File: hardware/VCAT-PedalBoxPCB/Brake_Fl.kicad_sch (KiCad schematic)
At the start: 7 parts, among them U4 INA241A5xD

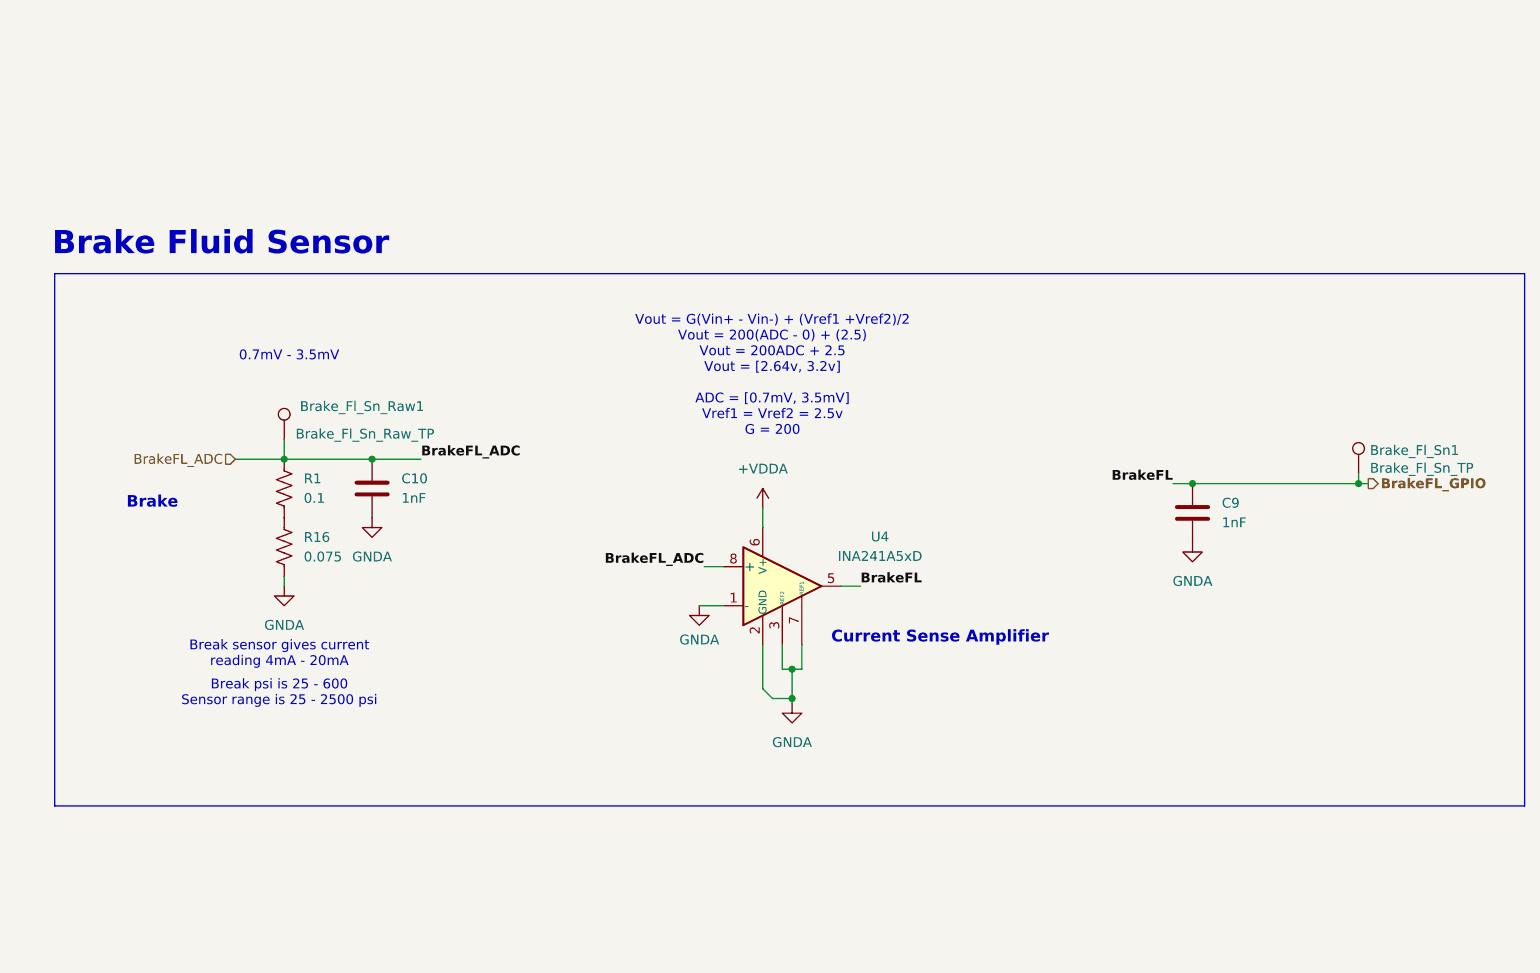
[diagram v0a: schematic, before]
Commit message: Rev B - Initial Layout
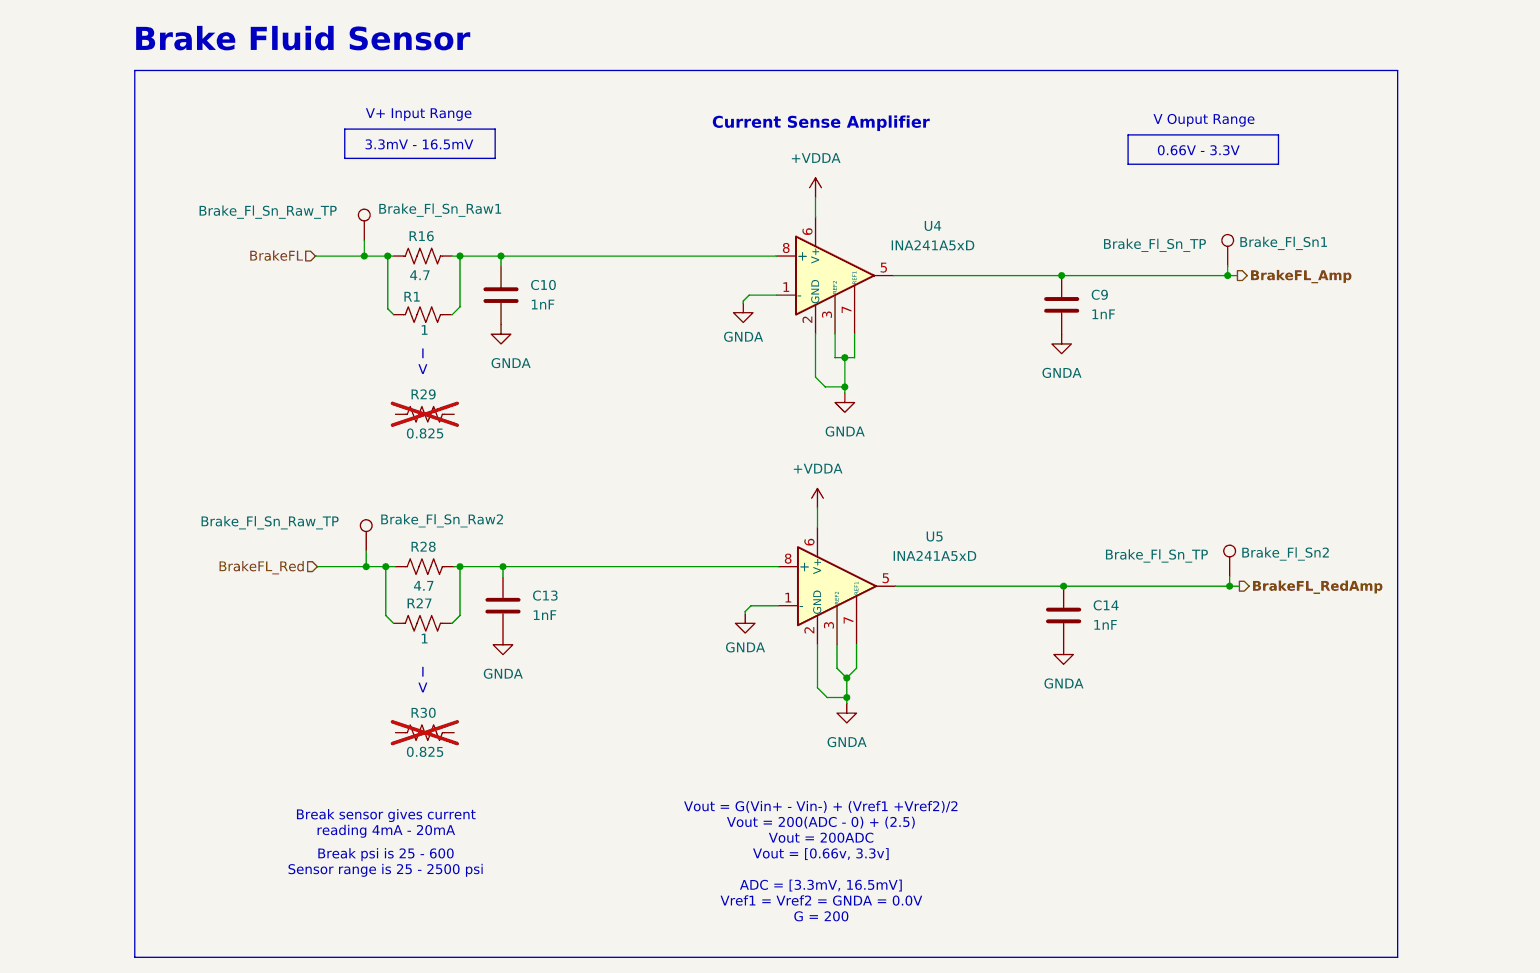
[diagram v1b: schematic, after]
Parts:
- added Brake_Fl_Sn2: Brake_Fl_Sn_TP, TestPoint:TestPoint_THTPad_1.5x1.5mm_Drill0.7mm, symbol Connector:TestPoint
- added Brake_Fl_Sn_Raw2: Brake_Fl_Sn_Raw_TP, TestPoint:TestPoint_THTPad_1.5x1.5mm_Drill0.7mm, symbol Connector:TestPoint
- added C13, C14: 1nF, Capacitor_SMD:C_0603_1608Metric_Pad1.08x0.95mm_HandSolder, symbol Device:C
- added R27: 1, Resistor_SMD:R_0603_1608Metric_Pad0.98x0.95mm_HandSolder, symbol Device:R_US
- added R28: 4.7, Resistor_SMD:R_0603_1608Metric_Pad0.98x0.95mm_HandSolder, symbol Device:R_US
- added R29, R30: 0.825, Resistor_SMD:R_0603_1608Metric_Pad0.98x0.95mm_HandSolder, symbol Device:R_US
- added U5: INA241A5xD, Package_SO:SOIC-8_3.9x4.9mm_P1.27mm, symbol Amplifier_Current:INA241A5xD
- R1: value 0.1 -> 1
- R16: value 0.075 -> 4.7
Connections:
- net +VDDA: now also U5.6 (V+)
- net GNDA: now also C13.2, C14.2, U5.1 (-), U5.2 (GND), U5.3 (REF2), U5.4 (GND), U5.7 (REF1); no longer R16.2
- net at R1.2: now also C10.1, R16.2, U4.8 (+); no longer R16.1
- net BrakeFL_ADC renamed BrakeFL
- net BrakeFL: now also R16.1; no longer C10.1, U4.8 (+)
- net BrakeFL_GPIO renamed BrakeFL_Amp
- new net: C13.1, R27.2, R28.2, U5.8 (+)
- new net BrakeFL_Red: Brake_Fl_Sn_Raw2.1, R27.1, R28.1
- new net BrakeFL_RedAmp: Brake_Fl_Sn2.1, C14.1, U5.5
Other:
- note added: "0.66V - 3.3V"
- note added: "3.3mV - 16.5mV"
- note added: "I V"
- note added: "V Ouput Range"
- note added: "V+ Input Range"
- note added: "Vout = G(Vin+ - Vin-) + (Vref1 +Vref2)/2 Vout = 200(ADC - 0) + (2.5) Vout = 200ADC Vout = [0.66v, 3.3v] ADC = [3.3mV, 16.5mV] Vref1 = Vref2 = GNDA = 0.0V G = 200"
- note removed: "0.7mV - 3.5mV"
- note removed: "Brake"
- note removed: "Vout = G(Vin+ - Vin-) + (Vref1 +Vref2)/2 Vout = 200(ADC - 0) + (2.5) Vout = 200ADC + 2.5 Vout = [2.64v, 3.2v] ADC = [0.7mV, 3.5mV] Vref1 = Vref2 = 2.5v G = 200"
- moved on the sheet: Brake_Fl_Sn1, Brake_Fl_Sn_Raw1, C10, C9, R1, R16, U4
